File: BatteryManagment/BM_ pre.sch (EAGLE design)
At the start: 74 parts, among them IC1 LMV321M5, U1 ATMEGA328P-AU, U2 LTC4440EMS8E-5PBF

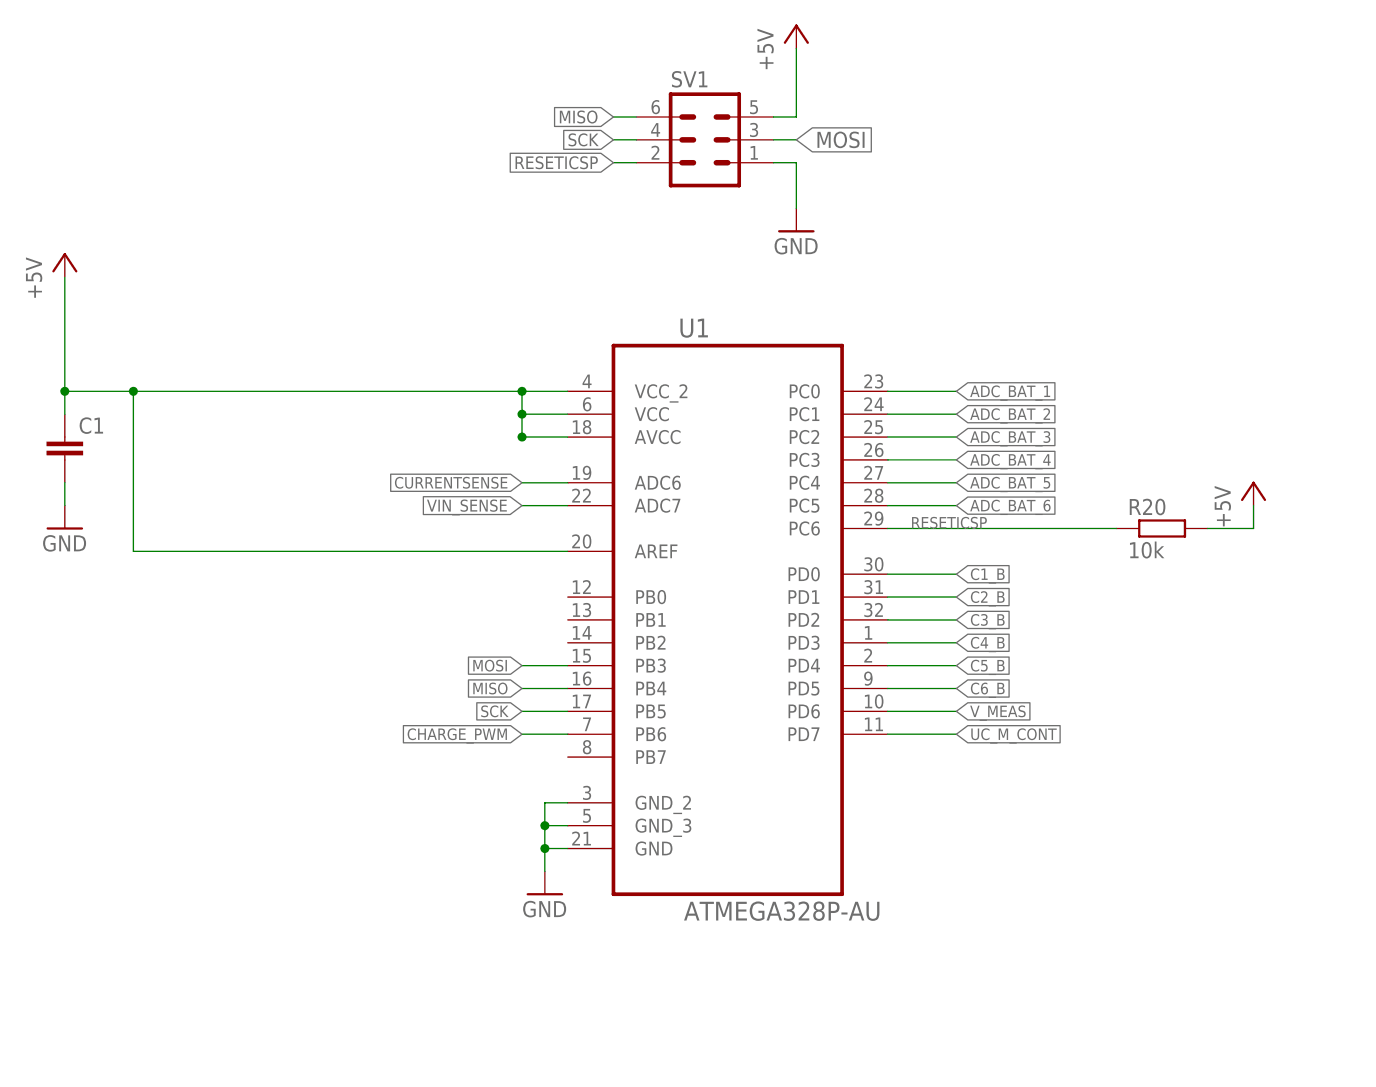
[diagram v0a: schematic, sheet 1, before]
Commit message: just updating my pc
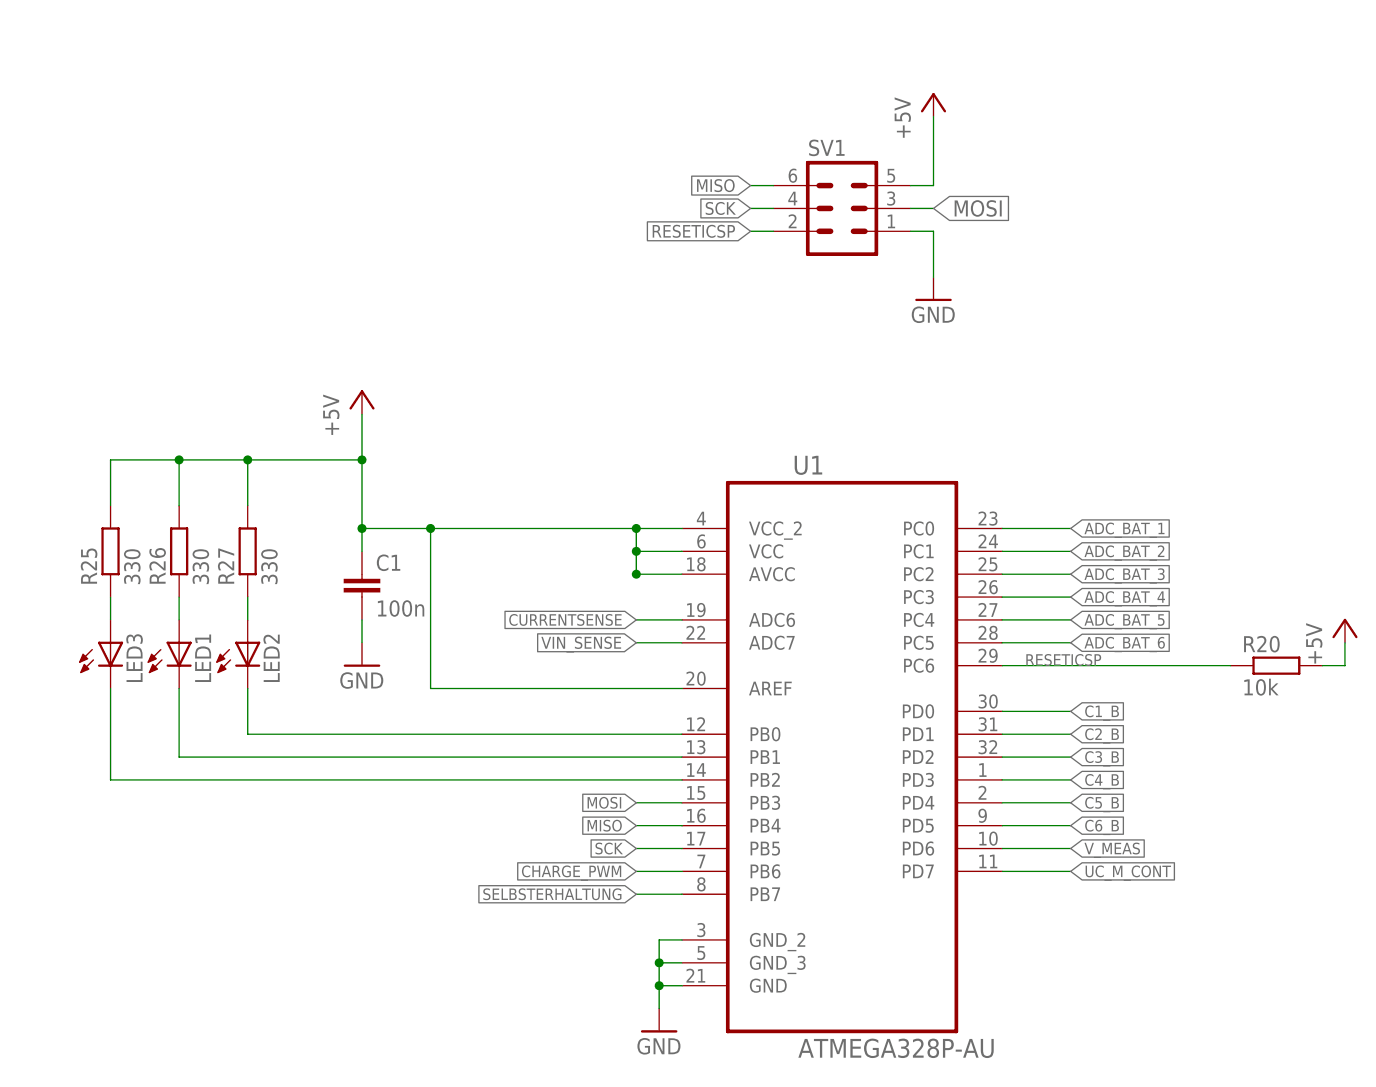
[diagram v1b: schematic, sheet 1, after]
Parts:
- removed R2: (no value), rcl:R-EU_R0603
- added LED1, LED2, LED3: (no value), eagle-ltspice:LED_E
- added PAD1, PAD2: (no value), wirepad:SMD5
- added R25, R26, R27: 330, rcl:R-EU_R0603
- added R28: (no value), rcl:R-EU_R0603
- added R29, R30: 1M, rcl:R-EU_R0603
- added U$22, U$23: IPB180P04P4L-02, BM_pre:IPB180P04P4L-02
- added U$24: FDN306P, BM_pre:FDN306P
- added U$25: FDN337N, BM_pre:FDN337N
- C1: value (none) -> 100n
- GND, VIN: value TPSQB2,54 -> Battery+; device testpad:TPSQB2,54 -> BM_pre:PAD
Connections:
- removed net N$3: R2.2, U$9.E
- new net N$17: LED2.C, U1.PB0
- new net N$18: LED1.C, U1.PB1
- new net N$19: LED3.C, U1.PB2
- new net N$20: PAD1.P, R29.1, U$24.G, U$25.D
- new net N$21: R29.2, U$24.S
- new net N$23: LED2.A, R27.1
- new net N$24: LED1.A, R26.1
- new net N$25: LED3.A, R25.1
- new net N$26: R28.1, U$21.C
- new net SELBSTERHALTUNG: R30.2, U$25.G, U1.PB7
- net +5V: now also R25.2, R26.2, R27.2
- net ADC_BAT_1: now also U$9.E; no longer R2.1
- net BATTERY+: now also U$22.S, U$23.S, U$24.D
- net GND: now also PAD2.P, R28.2, R30.1, U$25.S, U2.NC; no longer U$21.C
- net MOTOR+: now also U$22.D, U$23.D
- net MOTOR_CONTROL: now also U$22.G, U$23.G
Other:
- note added: "Taster"
- moved on the sheet: C1, C10, C11, C8, C9, R20, SV1, U$7, U$8, U1

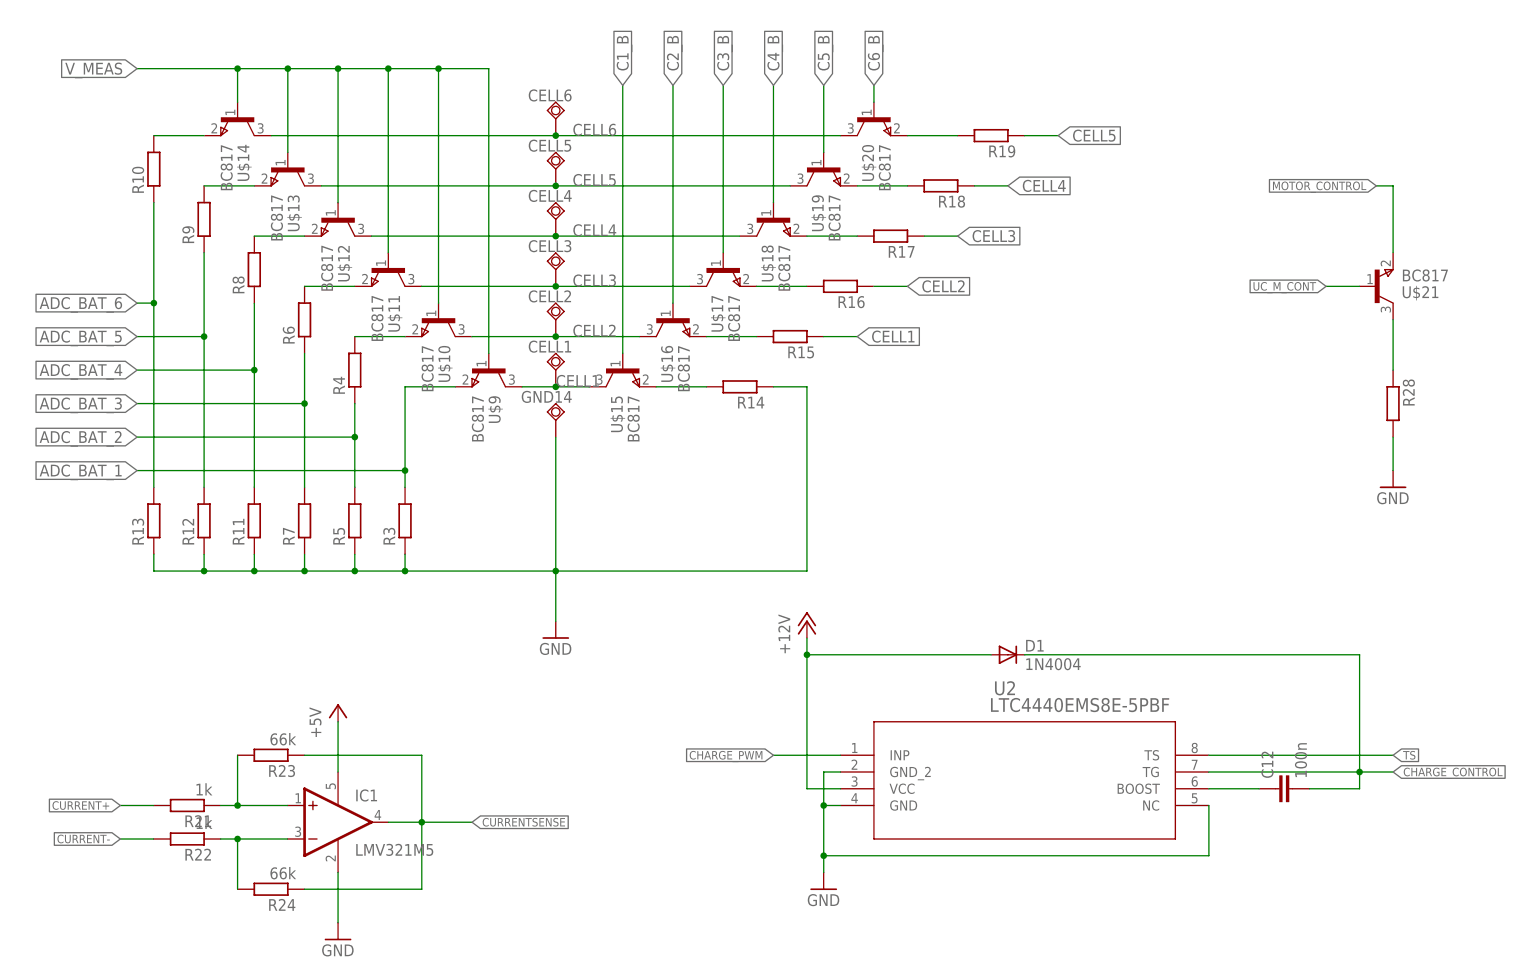
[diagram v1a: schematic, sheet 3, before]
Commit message: layout update
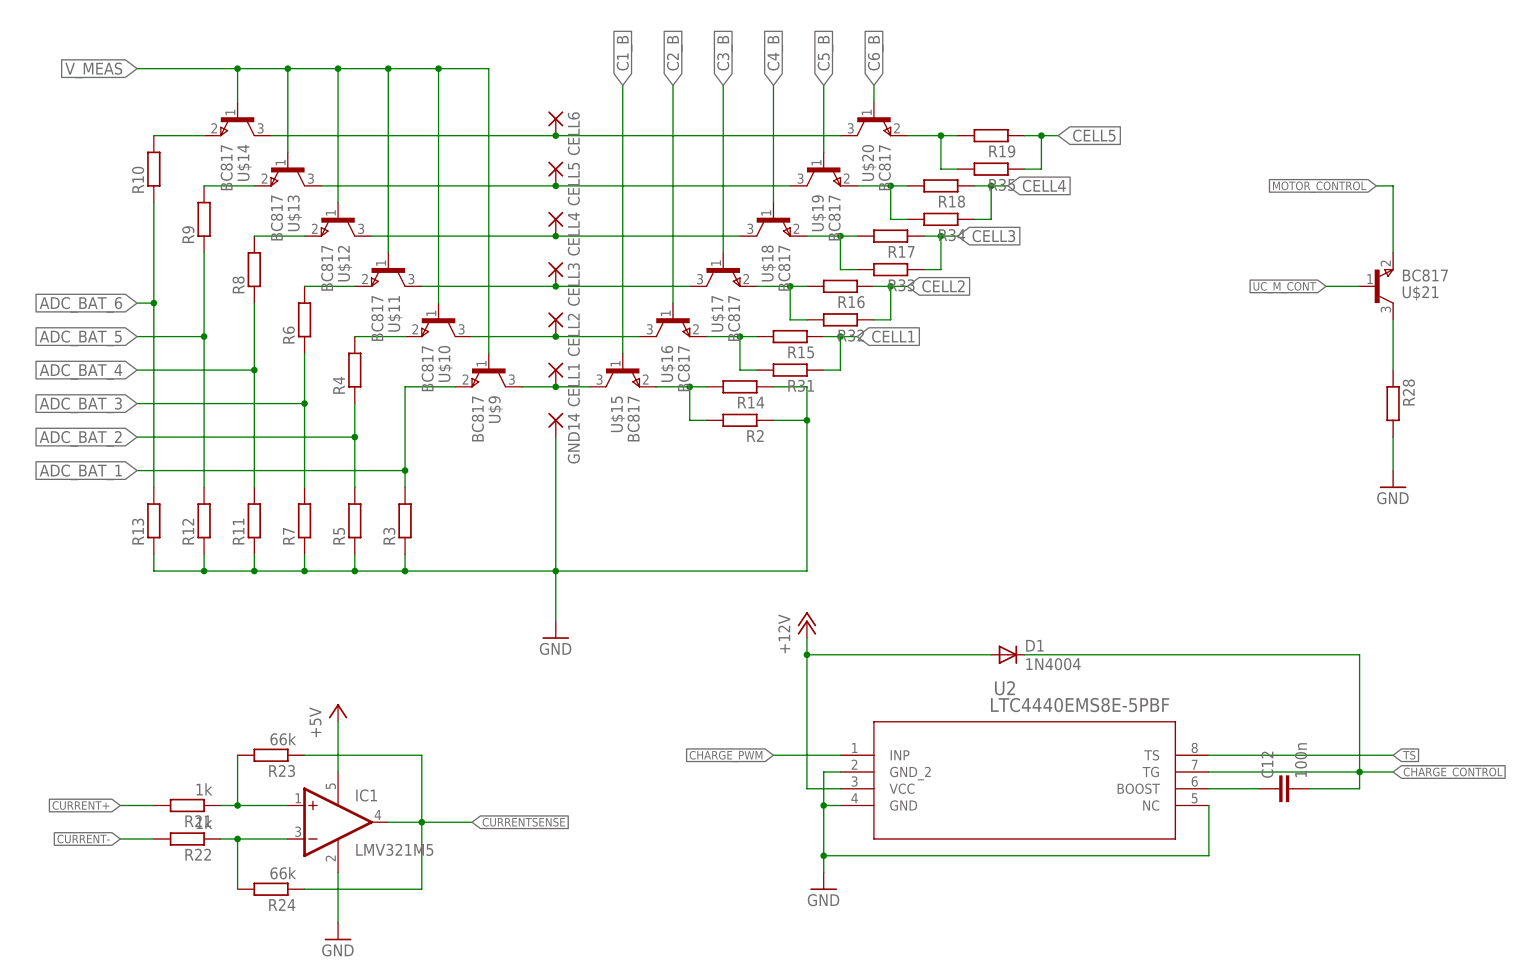
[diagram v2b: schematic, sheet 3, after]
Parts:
- added MOTOR+: Battery+, BM_pre:PAD
- added MOTOR-: PAD, BM_pre:PAD
- added R2, R31, R32, R33, R34, R35: (no value), rcl:R-EU_R0603
- BATTERY-: value PAD -> Battery+
- CELL1, CELL2, CELL3, CELL4, CELL5, CELL6, GND14: value TPSQB2,54 -> (none); device testpad:TPSQB2,54 -> wirepad:SMD5
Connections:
- net BATTERY+: now also BATTERY+.TP
- net CELL1: now also CELL1.P, R31.1; no longer CELL1.TP
- net CELL2: now also CELL2.P, R32.1; no longer CELL2.TP
- net CELL3: now also CELL3.P, R33.1; no longer CELL3.TP
- net CELL4: now also CELL4.P, R34.1; no longer CELL4.TP
- net CELL5: now also CELL5.P, R35.1; no longer CELL5.TP
- net CELL6: now also CELL6.P; no longer CELL6.TP
- net GND: now also GND14.P, MOTOR-.TP, R2.1; no longer GND14.TP
- net MOTOR+: now also MOTOR+.TP; no longer BATTERY+.TP
- net N$11: now also R32.2
- net N$12: now also R33.2
- net N$13: now also R34.2
- net N$14: now also R35.2
- net N$5: now also R2.2
- net N$6: now also R31.2
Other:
- moved on the sheet: BATTERY+, BATTERY-
